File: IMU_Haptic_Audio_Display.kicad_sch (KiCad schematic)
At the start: 24 parts, among them J2 Conn_01x02, J3 Conn_01x13, J4 Conn_01x02, U3 DRV2603, U4 LSM6DSOX, U6 SGTL5000

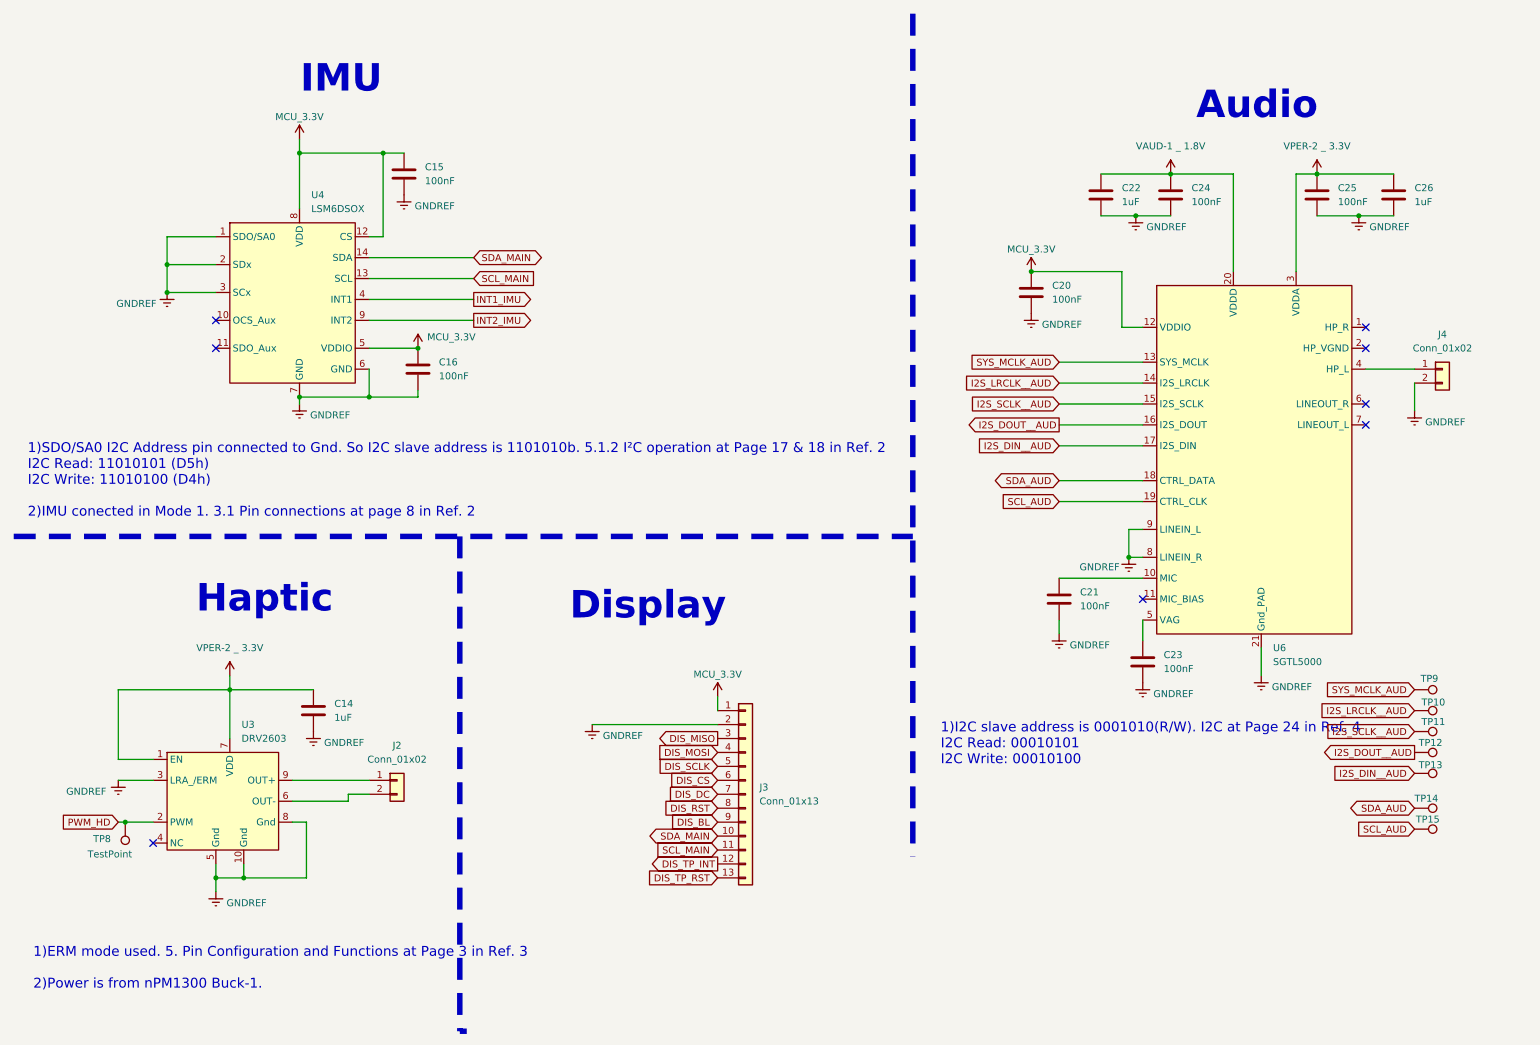
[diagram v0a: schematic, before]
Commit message: updated version
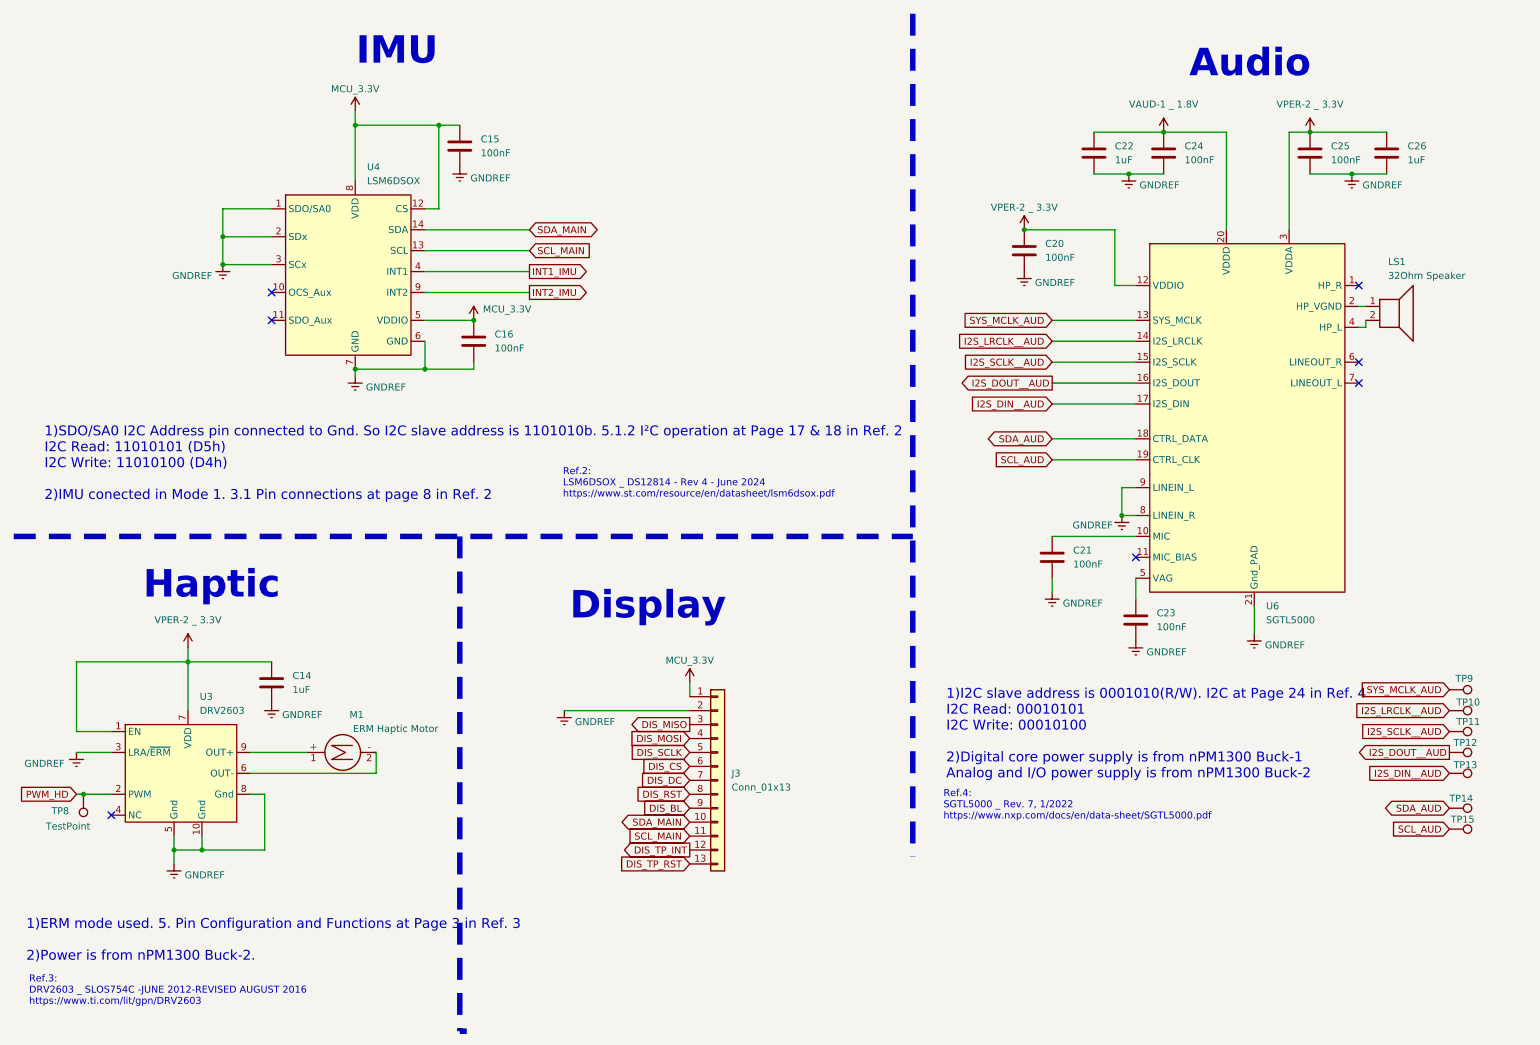
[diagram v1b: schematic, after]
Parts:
- removed J2, J4: Conn_01x02, Custom_Libs:2P_P1mm, symbol Connector_Generic:Conn_01x02
- added LS1: 32Ohm Speaker, symbol Device:Speaker
- added M1: ERM Haptic Motor, symbol Motor:Motor_DC
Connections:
- net MCU_3.3V: no longer C20.1, U6.12 (VDDIO)
- net VPER-2 _ 3.3V: now also C20.1, U6.12 (VDDIO)
- net at U3.6 (OUT-): now also M1.2 (-)
- net at U3.9 (OUT+): now also M1.1 (+)
- net at U6.4 (HP_L): now also LS1.2
- net at U6.2 (HP_VGND): now also LS1.1
- no-connect marks 8 -> 7
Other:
- note added: "1)ERM mode used. 5. Pin Configuration and Functions at Page 3 in Ref. 3 2)Power is from nPM1300 Buck-2."
- note added: "1)I2C slave address is 0001010(R/W). I2C at Page 24 in Ref. 4 I2C Read: 00010101 I2C Write: 00010100 2)Digital core power supply is from nPM1300 Buck-1 Analog and I/O power supply is from nPM1300 Buck-2"
- note added: "Ref.2: LSM6DSOX _ DS12814 - Rev 4 - June 2024 https://www.st.com/resource/en/datasheet/lsm6dsox.pdf"
- note added: "Ref.3: DRV2603 _ SLOS754C -JUNE 2012-REVISED AUGUST 2016 https://www.ti.com/lit/gpn/DRV2603"
- note added: "Ref.4: SGTL5000 _ Rev. 7, 1/2022 https://www.nxp.com/docs/en/data-sheet/SGTL5000.pdf"
- note removed: "1)ERM mode used. 5. Pin Configuration and Functions at Page 3 in Ref. 3 2)Power is from nPM1300 Buck-1."
- note removed: "1)I2C slave address is 0001010(R/W). I2C at Page 24 in Ref. 4 I2C Read: 00010101 I2C Write: 00010100"
- moved on the sheet: C14, C15, C16, C20, C21, C22, C23, C24, C25, C26, J3, TP10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
